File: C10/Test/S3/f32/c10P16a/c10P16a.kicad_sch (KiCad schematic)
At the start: 3 parts

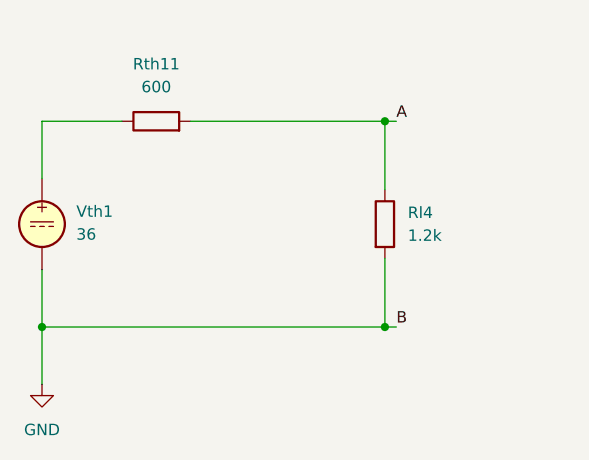
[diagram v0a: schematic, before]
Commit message: additional upload Chapter 10
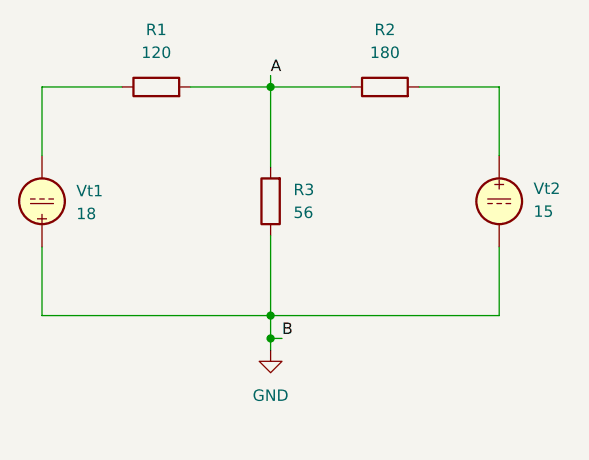
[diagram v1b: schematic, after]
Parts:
- removed Rl4: 1.2k, symbol Device:R
- removed Rth11: 600, symbol Device:R
- removed Vth1: 36, symbol Simulation_SPICE:VDC
- added R1: 120, symbol Device:R
- added R2: 180, symbol Device:R
- added R3: 56, symbol Device:R
- added Vt1: 18, symbol Simulation_SPICE:VDC
- added Vt2: 15, symbol Simulation_SPICE:VDC
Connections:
- net A: now also R1.2, R2.1, R3.2
- net GND: now also R3.1, Vt1.1, Vt2.2
- new net: R1.1, Vt1.2
- new net: R2.2, Vt2.1
